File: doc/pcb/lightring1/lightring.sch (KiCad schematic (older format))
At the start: 101 parts, among them J1 Conn_01x05_Female, SW1 SW_SPST, SW2 SW_SPST, U1 STM32G070RBT, Y1 Crystal

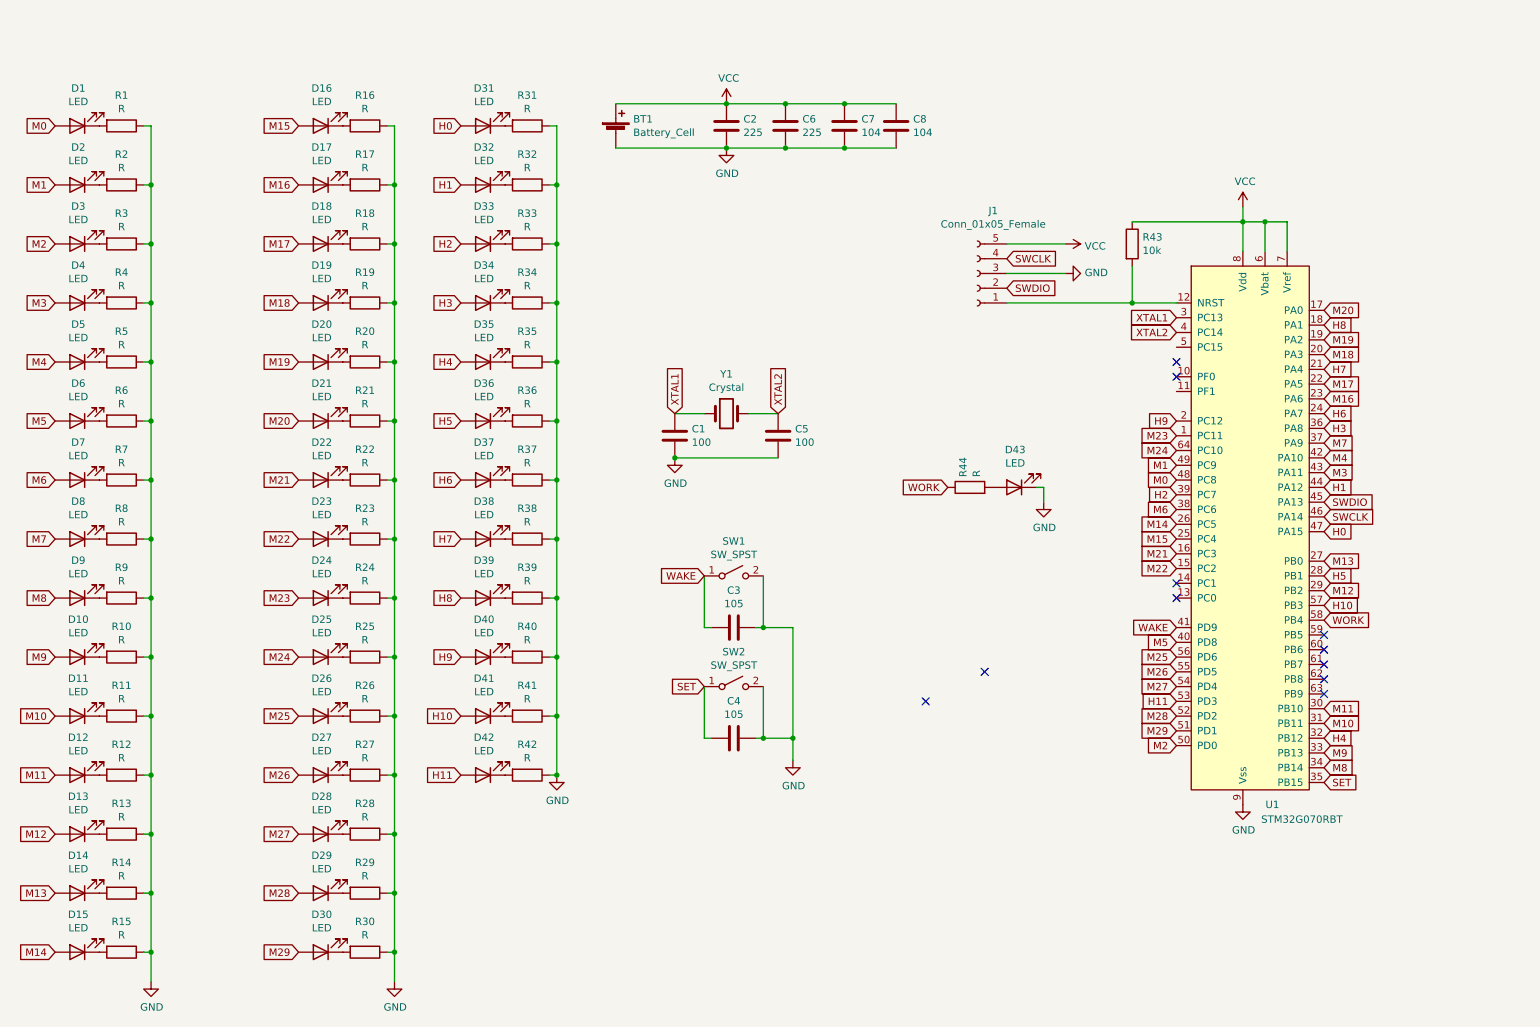
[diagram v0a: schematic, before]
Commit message: v0.2 board
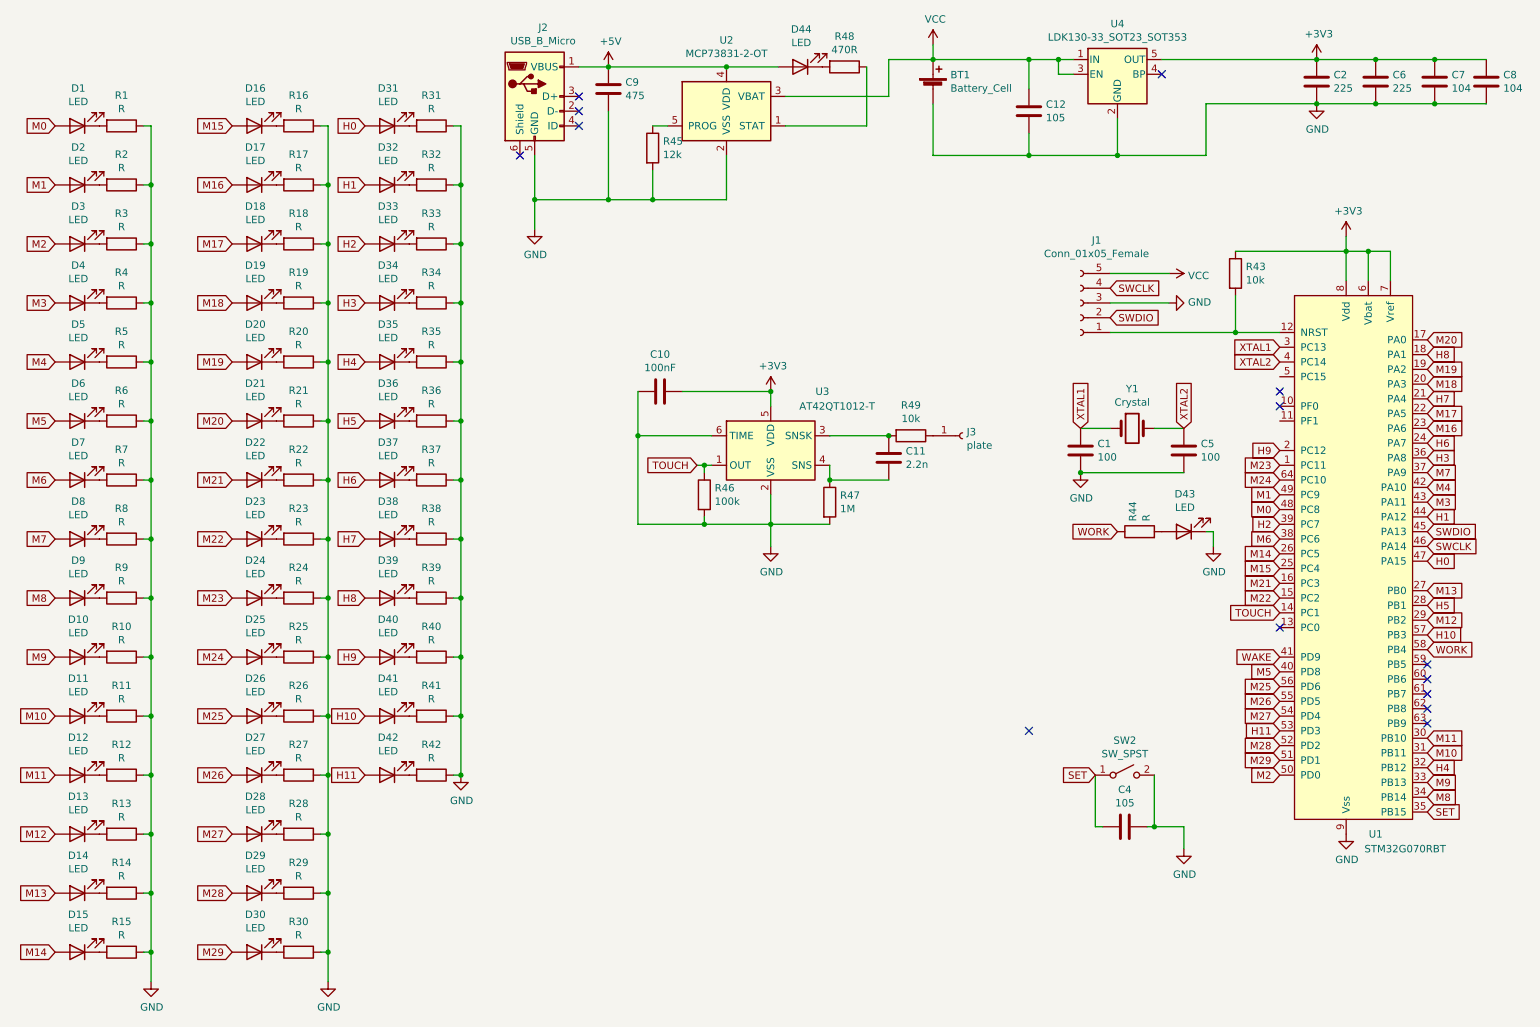
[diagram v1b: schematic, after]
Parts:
- removed C3: 105, lightring:LC_CAP, symbol Device:C
- removed SW1: SW_SPST, Button_Switch_SMD:Panasonic_EVQPUJ_EVQPUA, symbol Switch:SW_SPST
- added C10: 100nF, Capacitor_SMD:C_0603_1608Metric, symbol Device:C
- added C11: 2.2n, Capacitor_SMD:C_0603_1608Metric, symbol Device:C
- added C12: 105, Capacitor_SMD:C_0603_1608Metric, symbol Device:C
- added C9: 475, Capacitor_SMD:C_0603_1608Metric, symbol Device:C
- added D44: LED, Diode_SMD:D_0603_1608Metric, symbol Device:LED
- added J2: USB_B_Micro, Connector_USB:USB_Micro-B_Molex_47346-0001, symbol Connector:USB_B_Micro
- added J3: plate, lightring:touchplate, symbol Connector:Conn_01x01_Female
- added R45: 12k, Resistor_SMD:R_0603_1608Metric, symbol Device:R
- added R46: 100k, Resistor_SMD:R_0603_1608Metric, symbol Device:R
- added R47: 1M, Resistor_SMD:R_0603_1608Metric, symbol Device:R
- added R48: 470R, Resistor_SMD:R_0603_1608Metric, symbol Device:R
- added R49: 10k, Resistor_SMD:R_0603_1608Metric, symbol Device:R
- added U2: MCP73831-2-OT, Package_TO_SOT_SMD:SOT-23-5, symbol Battery_Management:MCP73831-2-OT
- added U3: AT42QT1012-T, Package_TO_SOT_SMD:SOT-23-6, symbol Sensor_Touch:AT42QT1012-T
- added U4: LDK130-33_SOT23_SOT353, Package_TO_SOT_SMD:SOT-23-5, symbol Regulator_Linear:LDK130-33_SOT23_SOT353
- BT1: footprint Battery:BatteryHolder_Keystone_500 -> Resistor_SMD:R_1206_3216Metric
- C1, C2, C4, C5, C6, C7, C8: footprint lightring:LC_CAP -> Capacitor_SMD:C_0603_1608Metric
- R43, R44: footprint lightring:LR_RES -> Resistor_SMD:R_0603_1608Metric
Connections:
- net GND: now also C10.2, C12.2, C9.2, J2.5 (GND), R45.2, R46.2, R47.2, U2.2 (VSS), U3.2 (VSS), U3.6 (TIME), U4.2 (GND)
- net VCC: now also C12.1, U2.3 (VBAT), U4.1 (IN), U4.3 (EN); no longer C2.1, C6.1, C7.1, C8.1, R43.1, U1.6 (Vbat), U1.7 (Vref), U1.8 (Vdd)
- net TOUCH: now reaches U1.14 (PC1)
- net TOUCH: now also R46.1, U3.1 (OUT)
- new net: R48.1, U2.1 (STAT)
- new net: R45.1, U2.5 (PROG)
- new net: D44.1 (K), R48.2
- new net: C11.1, R49.2, U3.3 (SNSK)
- new net: C11.2, R47.1, U3.4 (SNS)
- new net: J3.1 (Pin_1), R49.1
- new net +3V3: C10.1, C2.1, C6.1, C7.1, C8.1, R43.1, U1.6 (Vbat), U1.7 (Vref), U1.8 (Vdd), U3.5 (VDD), U4.5 (OUT)
- new net +5V: C9.1, D44.2 (A), J2.1 (VBUS), U2.4 (VDD)
- no-connect marks 11 -> 14
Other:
- moved on the sheet: BT1, C1, C2, C4, C5, C6, C7, C8, D16, D17, D18, D19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
